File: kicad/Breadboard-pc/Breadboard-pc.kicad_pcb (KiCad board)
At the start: 2 copper layers, 117.5 x 84.5 mm, 11 parts, among them U1 8088, U11 8255A, U3 74HC573, U4 W29C020C, U6 74HC245, U7 74HC573, U8 HM628128D, U9 74HCT00

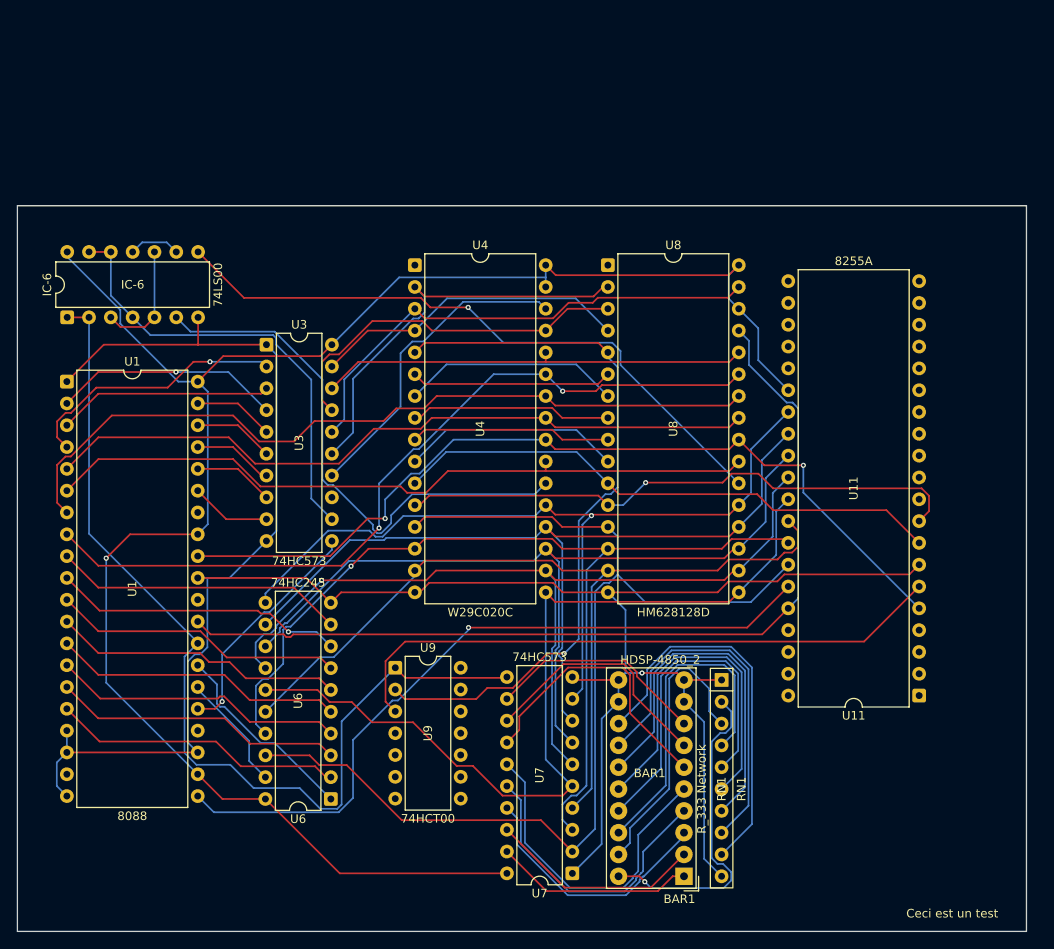
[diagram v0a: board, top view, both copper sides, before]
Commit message: Actualisé le PCB
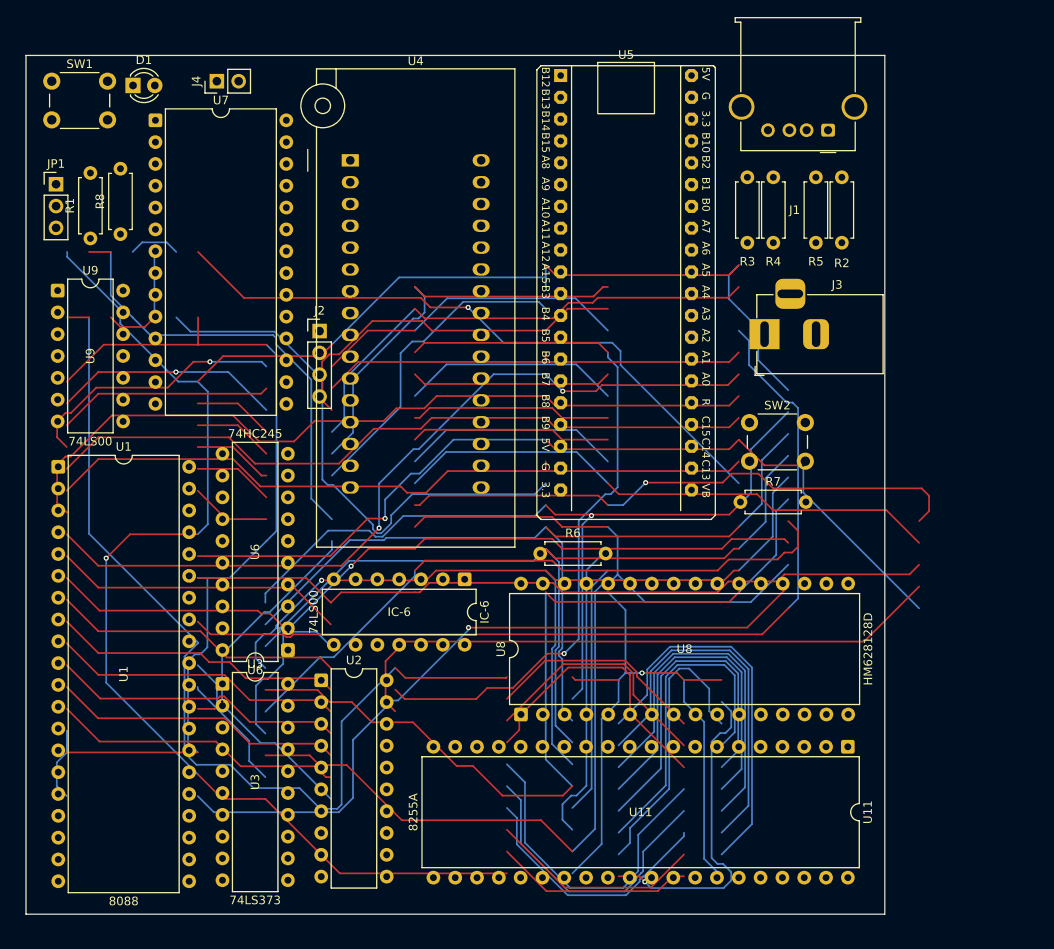
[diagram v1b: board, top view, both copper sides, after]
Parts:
- removed BAR1: HDSP-4850_2, Display:HDSP-4850
- removed RN1: R_333 Network, Resistor_THT:R_Array_SIP10
- added D1: PWR, LED_THT:LED_D3.0mm, F.Cu at (104.0, 42.0)
- added J1: USB_A (clavier PS/2), Connector_USB:USB_A_Molex_67643_Horizontal, F.Cu at (184.9, 47.2)
- added J2: LCD I2C, Connector_PinHeader_2.54mm:PinHeader_1x04_P2.54mm_Vertical, F.Cu at (125.7, 70.6)
- added J3: 5V 2A, Connector_BarrelJack:BarrelJack_Horizontal, F.Cu at (177.5, 71.0)
- added J4: CLK externe, Connector_PinHeader_2.54mm:PinHeader_1x02_P2.54mm_Vertical, F.Cu at (113.7, 41.5)
- added JP1: 1-2: STM32 2-3: ext., Connector_PinHeader_2.54mm:PinHeader_1x03_P2.54mm_Vertical, F.Cu at (95.0, 53.5)
- added R1: 4.7k, Resistor_THT:R_Axial_DIN0207_L6.3mm_D2.5mm_P7.62mm_Horizontal, F.Cu at (99.0, 59.8)
- added R2: 10k, Resistor_THT:R_Axial_DIN0207_L6.3mm_D2.5mm_P7.62mm_Horizontal, F.Cu at (186.5, 60.3)
- added R3: 10k, Resistor_THT:R_Axial_DIN0207_L6.3mm_D2.5mm_P7.62mm_Horizontal, F.Cu at (175.5, 60.3)
- added R4: 10k, Resistor_THT:R_Axial_DIN0207_L6.3mm_D2.5mm_P7.62mm_Horizontal, F.Cu at (178.5, 60.3)
- added R5: 4.7k, Resistor_THT:R_Axial_DIN0207_L6.3mm_D2.5mm_P7.62mm_Horizontal, F.Cu at (183.5, 60.3)
- added R6: 4.7k, Resistor_THT:R_Axial_DIN0207_L6.3mm_D2.5mm_P7.62mm_Horizontal, F.Cu at (151.4, 96.5)
- added R7: 10k, Resistor_THT:R_Axial_DIN0207_L6.3mm_D2.5mm_P7.62mm_Horizontal, F.Cu at (174.7, 90.5)
- added R8: 1k, Resistor_THT:R_Axial_DIN0207_L6.3mm_D2.5mm_P7.62mm_Horizontal, F.Cu at (102.5, 59.3)
- added SW1: RESET, Button_Switch_THT:SW_PUSH_6mm, F.Cu at (94.5, 41.5)
- added SW2: IR0 test, Button_Switch_THT:SW_PUSH_6mm, F.Cu at (175.8, 81.2)
- added U2: 74LS373, Package_DIP:DIP-20_W7.62mm, F.Cu at (125.9, 111.3)
- added U5: STM32F411 BlackPill, Black-Pill:STM32F411_Black_Pill, F.Cu at (161.4, 65.0)
- U3: value 74HC573 -> 74LS373
- U4: footprint Package_DIP:DIP-32_W15.24mm -> Socket:DIP_Socket-32_W11.9mm_W12.7mm_W15.24mm_W17.78mm_W18.5mm_3M_232-1285-00-0602J
- U7: value 74HC573 -> 8259A; footprint Package_DIP:DIP-20_W7.62mm -> Package_DIP:DIP-28_W15.24mm
- U9: value 74HCT00 -> 74LS00
- moved U7 100.2 mm to (106.6, 46.1), turned to 0 degrees
- moved U9 58.9 mm to (95.2, 65.9)
- moved IC-6 55.4 mm to (142.6, 99.5), turned to -90 degrees
- moved U8 53.3 mm to (149.1, 115.2), turned to 90 degrees
- moved U3 39.8 mm to (114.4, 111.7)
- moved U6 18.0 mm to (122.0, 107.7)
- moved U4 14.3 mm to (129.3, 50.7)
- moved U11 10.2 mm to (187.2, 119.0), turned to -90 degrees
- moved U1 9.97 mm to (95.3, 86.4)
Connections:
- net /A7 renamed A7
- net /CS8255_ renamed CS8255_
- net /RESET renamed RESET
- IC-6 pad 1: /<NO NET> -> IO
- IC-6 pad 12: /A19 -> A19
- IC-6 pad 13: /A19 -> A19
- IC-6 pad 2: /<NO NET> -> IO
- IC-6 pad 4: /A19 -> A19
- U1 pad 18: GND -> /INTR
- U1 pad 19: unconnected-(U1-CLK-Pad19) -> CLK
- U1 pad 24: unconnected-(U1-~{INTA}-Pad24) -> /INTA_
- U1 pad 28: /<NO NET> -> IO
- U11 pad 1: unconnected-(U11-PA3-Pad1) -> /BUS_PA3
- U11 pad 10: unconnected-(U11-PC7-Pad10) -> /OBF_
- U11 pad 11: unconnected-(U11-PC6-Pad11) -> /ACK_
- U11 pad 12: unconnected-(U11-PC5-Pad12) -> /IBF
- U11 pad 13: unconnected-(U11-PC4-Pad13) -> /STB_
- U11 pad 14: unconnected-(U11-PC0-Pad14) -> /TAG
- U11 pad 15: unconnected-(U11-PC1-Pad15) -> /TAG1
- U11 pad 17: unconnected-(U11-PC3-Pad17) -> /IRQ1
- U11 pad 18: unconnected-(U11-PB0-Pad18) -> /CANAL0
- U11 pad 19: unconnected-(U11-PB1-Pad19) -> /CANAL1
- U11 pad 2: unconnected-(U11-PA2-Pad2) -> /BUS_PA2
- U11 pad 3: unconnected-(U11-PA1-Pad3) -> /BUS_PA1
- U11 pad 37: unconnected-(U11-PA7-Pad37) -> /BUS_PA7
- U11 pad 38: unconnected-(U11-PA6-Pad38) -> /BUS_PA6
- U11 pad 39: unconnected-(U11-PA5-Pad39) -> /BUS_PA5
- U11 pad 4: unconnected-(U11-PA0-Pad4) -> /BUS_PA0
- U11 pad 40: unconnected-(U11-PA4-Pad40) -> /BUS_PA4
- U3 pad 12: /A19 -> /A16
- U3 pad 13: /A18 -> Net-(U1-A16/S3)
- U3 pad 14: /A17 -> Net-(U1-A17/S4)
- U3 pad 15: /A16 -> /A17
- U3 pad 16: /A15 -> /A18
- U3 pad 17: /A14 -> Net-(U1-A18/S5)
- U3 pad 18: /A13 -> Net-(U1-A19/S6)
- U3 pad 19: /A12 -> A19
- U3 pad 2: Net-(U1-A12) -> /A12
- U3 pad 3: Net-(U1-A13) -> Net-(U1-A12)
- U3 pad 4: Net-(U1-A14) -> Net-(U1-A13)
- U3 pad 5: Net-(U1-A15) -> /A13
- U3 pad 6: Net-(U1-A16/S3) -> /A14
- U3 pad 7: Net-(U1-A17/S4) -> Net-(U1-A14)
- U3 pad 8: Net-(U1-A18/S5) -> Net-(U1-A15)
- U3 pad 9: Net-(U1-A19/S6) -> /A15
- U7 pad 1: GND -> /CS8259_
- U7 pad 10: GND -> /D1
- U7 pad 11: /<NO NET> -> /D0
- U7 pad 12: Net-(U7-Q7) -> unconnected-(U7-CAS0-Pad12)
- U7 pad 13: Net-(U7-Q6) -> unconnected-(U7-CAS1-Pad13)
- U7 pad 14: Net-(U7-Q5) -> GND
- U7 pad 15: Net-(U7-Q4) -> unconnected-(U7-CAS2-Pad15)
- U7 pad 16: Net-(U7-Q3) -> +5V
- U7 pad 17: Net-(U7-Q2) -> /INTR
- U7 pad 19: Net-(U7-Q0) -> /IRQ1
- U7 pad 2: /D0 -> /WR_
- U7 pad 20: +5V -> GND
- U7 pad 3: /D1 -> /RD_
- U7 pad 4: /D2 -> /D7
- U7 pad 5: /D3 -> /D6
- U7 pad 6: /D4 -> /D5
- U7 pad 7: /D5 -> /D4
- U7 pad 8: /D6 -> /D3
- U7 pad 9: /D7 -> /D2
- U9 pad 1: /<NO NET> -> IO
- U9 pad 14: (no net) -> +5V
- U9 pad 4: (no net) -> IO
- U9 pad 5: (no net) -> /A5
- U9 pad 6: (no net) -> /CS8259_
- U9 pad 7: (no net) -> GND
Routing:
- net (no net): track 0.00 -> 429.4 mm, vias 0 -> 1
- net /D3: track 101.8 -> 355.5 mm
- net /A6: track 23.4 -> 243.1 mm
- net /<NO NET>: track 112.4 -> 0.00 mm
- net IO: track 0.00 -> 96.3 mm
- net unconnected-(U5-VBat-Pad21): track 0.00 -> 95.7 mm, vias 0 -> 1
- net Net-(IC-6-Pad10): track 13.6 -> 105.3 mm
- net RESET: track 84.5 -> 0.00 mm
- net /A10: track 84.0 -> 0.00 mm
- net /A1: track 64.6 -> 0.00 mm
- net /ROM/SEL: track 63.5 -> 0.00 mm
- net GND: track 273.5 -> 217.2 mm
- net /D4: track 101.6 -> 157.9 mm
- net /RD_: track 101.8 -> 47.4 mm, vias 2 -> 1
- net /A19: track 52.7 -> 0.00 mm
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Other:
- board size 117.5 x 84.5 mm -> 100 x 100 mm
- board text removed: "Ceci est un test"
